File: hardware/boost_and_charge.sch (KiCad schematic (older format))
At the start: 37 parts, among them J1 Conn_01x02_Female, J4 Conn_01x02_Male, SW5 SW_Push, U4 MCP73871, U5 TPS61090

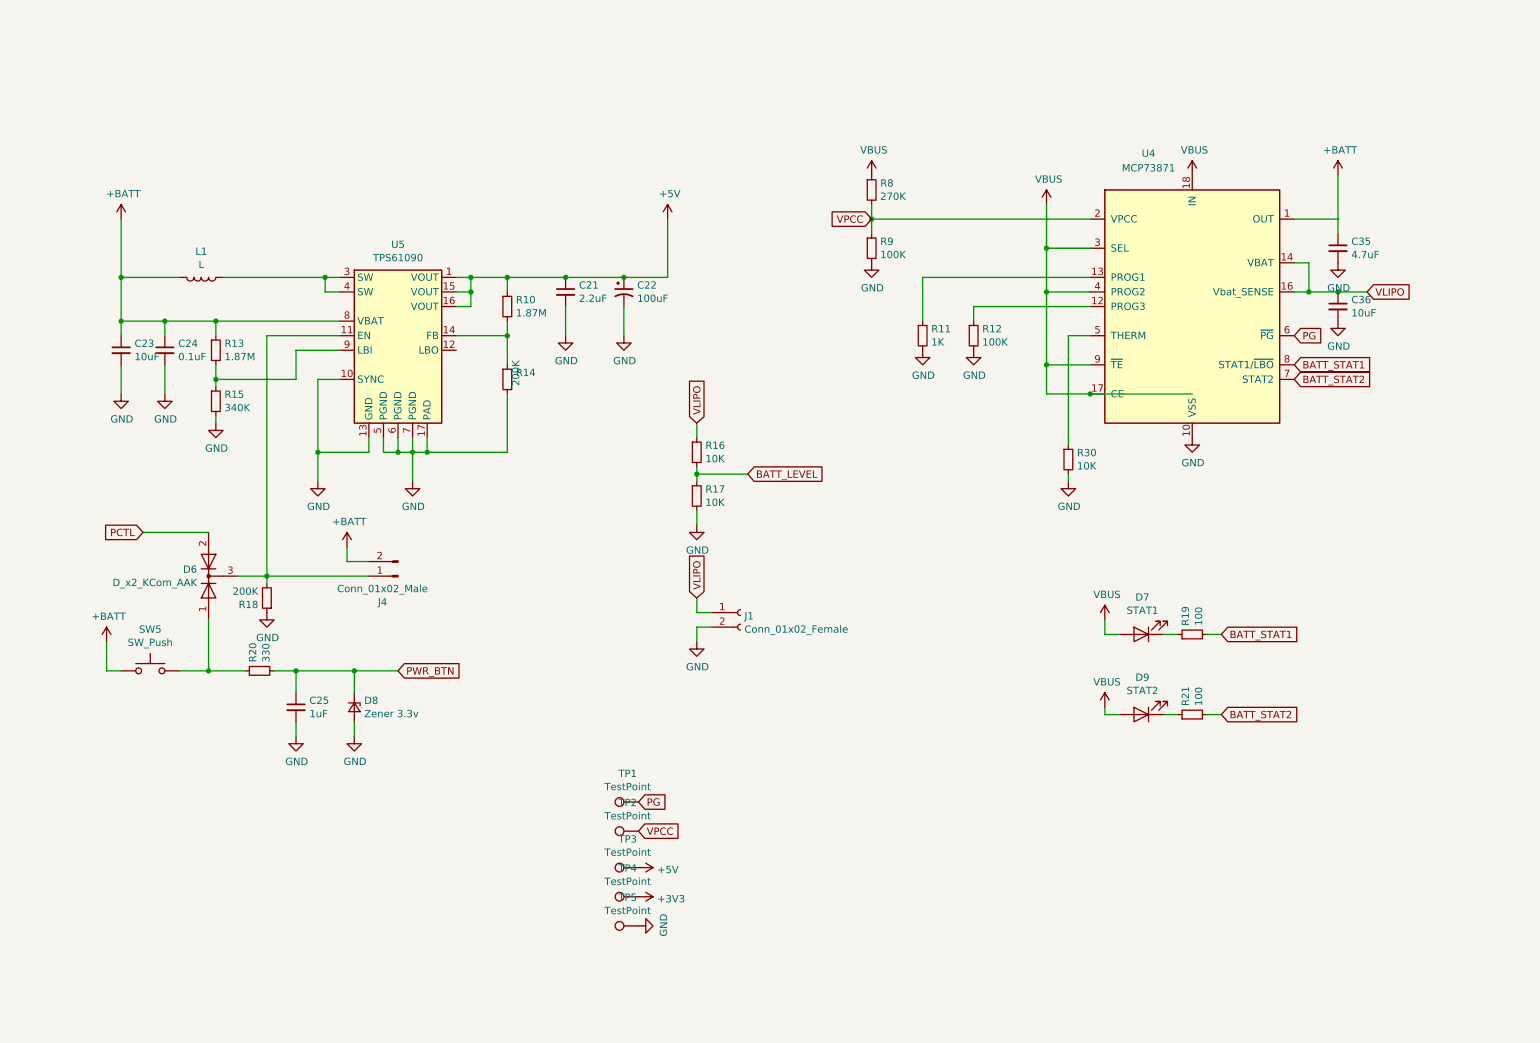
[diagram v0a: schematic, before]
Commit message: v2 mostly routed
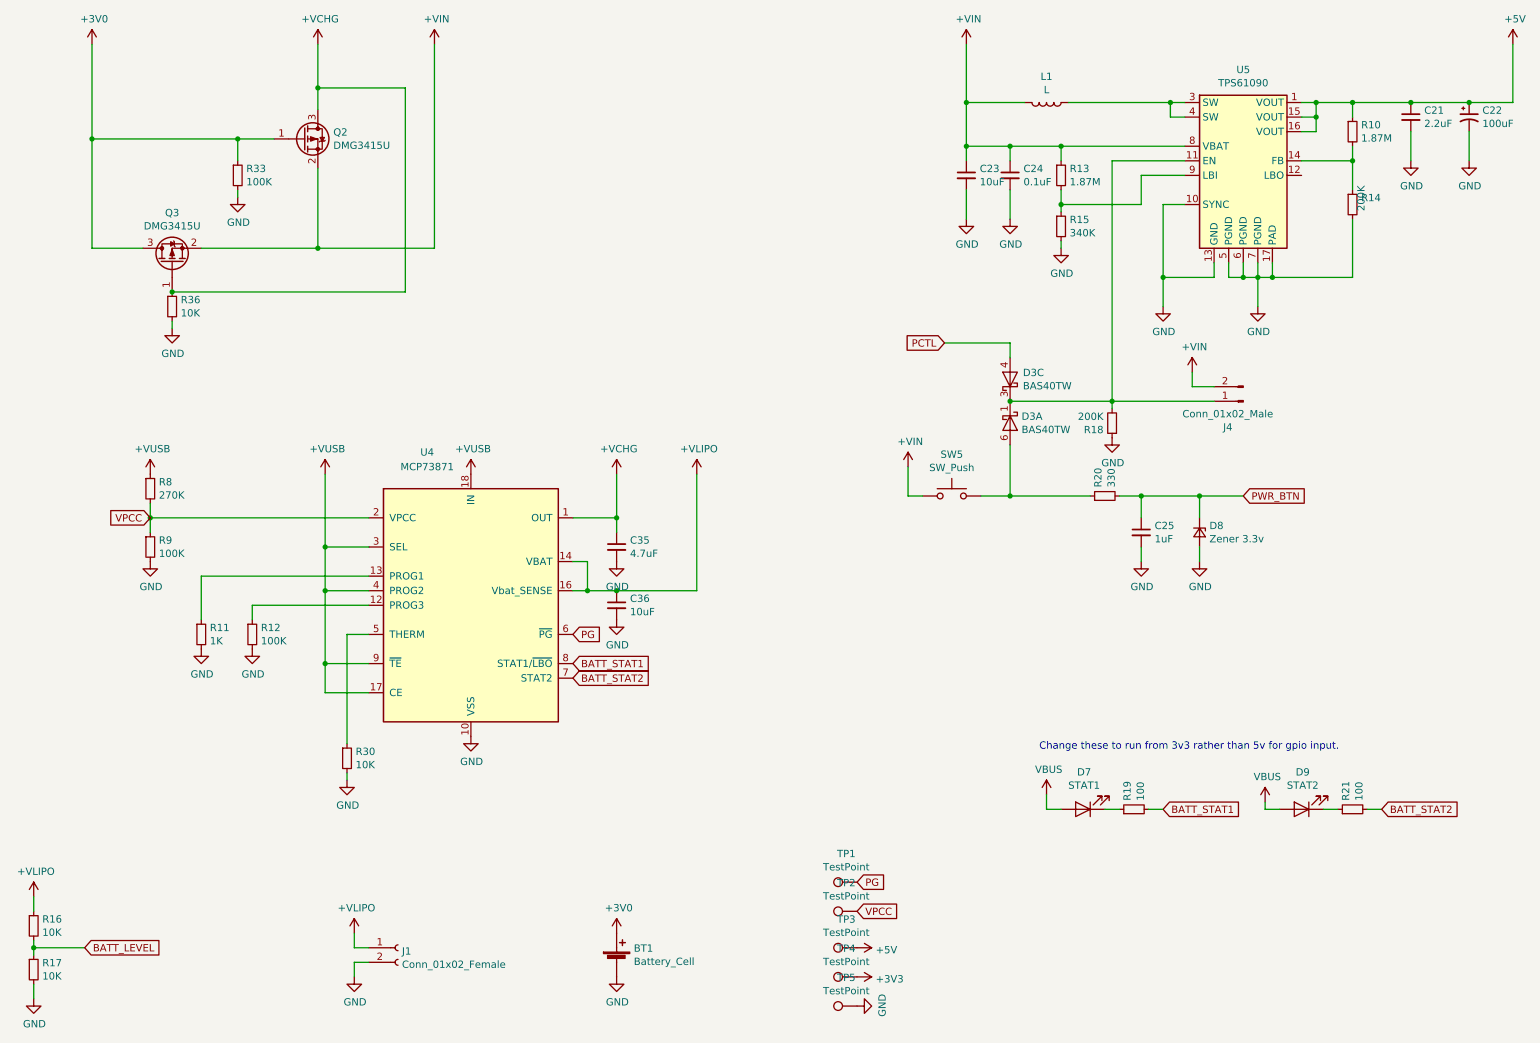
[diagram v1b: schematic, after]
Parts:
- removed D6: D_x2_KCom_AAK, digikey-footprints:SOT-23-3, symbol Device:D_x2_KCom_AAK
- added BT1: Battery_Cell, Battery:BatteryHolder_Keystone_2462_2xAA, symbol Device:Battery_Cell
- added D3: BAS40TW, Package_TO_SOT_SMD:SOT-363_SC-70-6, symbol teensy_beats-rescue:BAS40TW-teensy_beats_parts
- added Q2, Q3: DMG3415U, Package_TO_SOT_SMD:SOT-23, symbol Transistor_FET:DMG2301L
- added R33: 100K, Resistor_SMD:R_0402_1005Metric, symbol Device:R_Small
- added R36: 10K, Resistor_SMD:R_0402_1005Metric, symbol Device:R_Small
- C21, C23, C25, C35, C36: footprint Capacitors_SMD:C_0805 -> Capacitor_SMD:C_0805_2012Metric
- C22: footprint Capacitors_SMD:C_1210 -> Capacitor_SMD:C_1210_3225Metric
- C24: footprint Capacitors_SMD:C_0805 -> Capacitor_SMD:C_0402_1005Metric
- R10, R11, R12, R13, R14, R15, R16, R17, R18, R19, R20, R21, R30, R8, R9: footprint Resistors_SMD:R_0805 -> Resistor_SMD:R_0402_1005Metric
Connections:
- net GND: now also BT1.2 (-), R33.2, R36.2
- net PCTL: now also D3.4 (A)
- net VBUS: no longer R8.1, U4.17 (CE), U4.18 (IN), U4.19 (IN), U4.3 (SEL), U4.4 (PROG2), U4.9 (~TE)
- net at R20.1, SW5.1: now also D3.6 (A)
- net at J4.1 (Pin_1), R18.2, U5.11 (EN): now also D3.1 (K), D3.3 (K)
- net +BATT renamed +VIN
- net +VIN: now also Q2.2 (S), Q3.2 (S); no longer C35.1, U4.1 (OUT), U4.20 (OUT)
- net VLIPO renamed +VLIPO
- new net +3V0: BT1.1 (+), Q2.1 (G), Q3.3 (D), R33.1
- new net +VCHG: C35.1, Q2.3 (D), Q3.1 (G), R36.1, U4.1 (OUT), U4.20 (OUT)
- new net +VUSB: R8.1, U4.17 (CE), U4.18 (IN), U4.19 (IN), U4.3 (SEL), U4.4 (PROG2), U4.9 (~TE)
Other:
- note added: "Change these to run from 3v3 rather than 5v for gpio input."
- moved on the sheet: C21, C22, C23, C24, C25, C35, C36, D7, D8, D9, J1, J4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
